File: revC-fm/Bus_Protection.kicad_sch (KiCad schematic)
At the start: 79 parts, among them Q24 MMDT2907AQ-7-F, Q25 MMDT5551-7-F, Q26 MMDT5551-7-F, Q27 MMDT5551-7-F, Q28 MMDT5551-7-F, Q29 MMDT2907AQ-7-F, Q30 BSS138DWQ-7, Q31 BSS138DWQ-7, Q32 BSS138DWQ-7, Q33 BSS138DWQ-7, Q34 MMDT3946, Q34 MMDT5551-7-F, Q35 MMDT5551-7-F, Q37 BSS138DWQ-7, Q38 BSS138DWQ-7

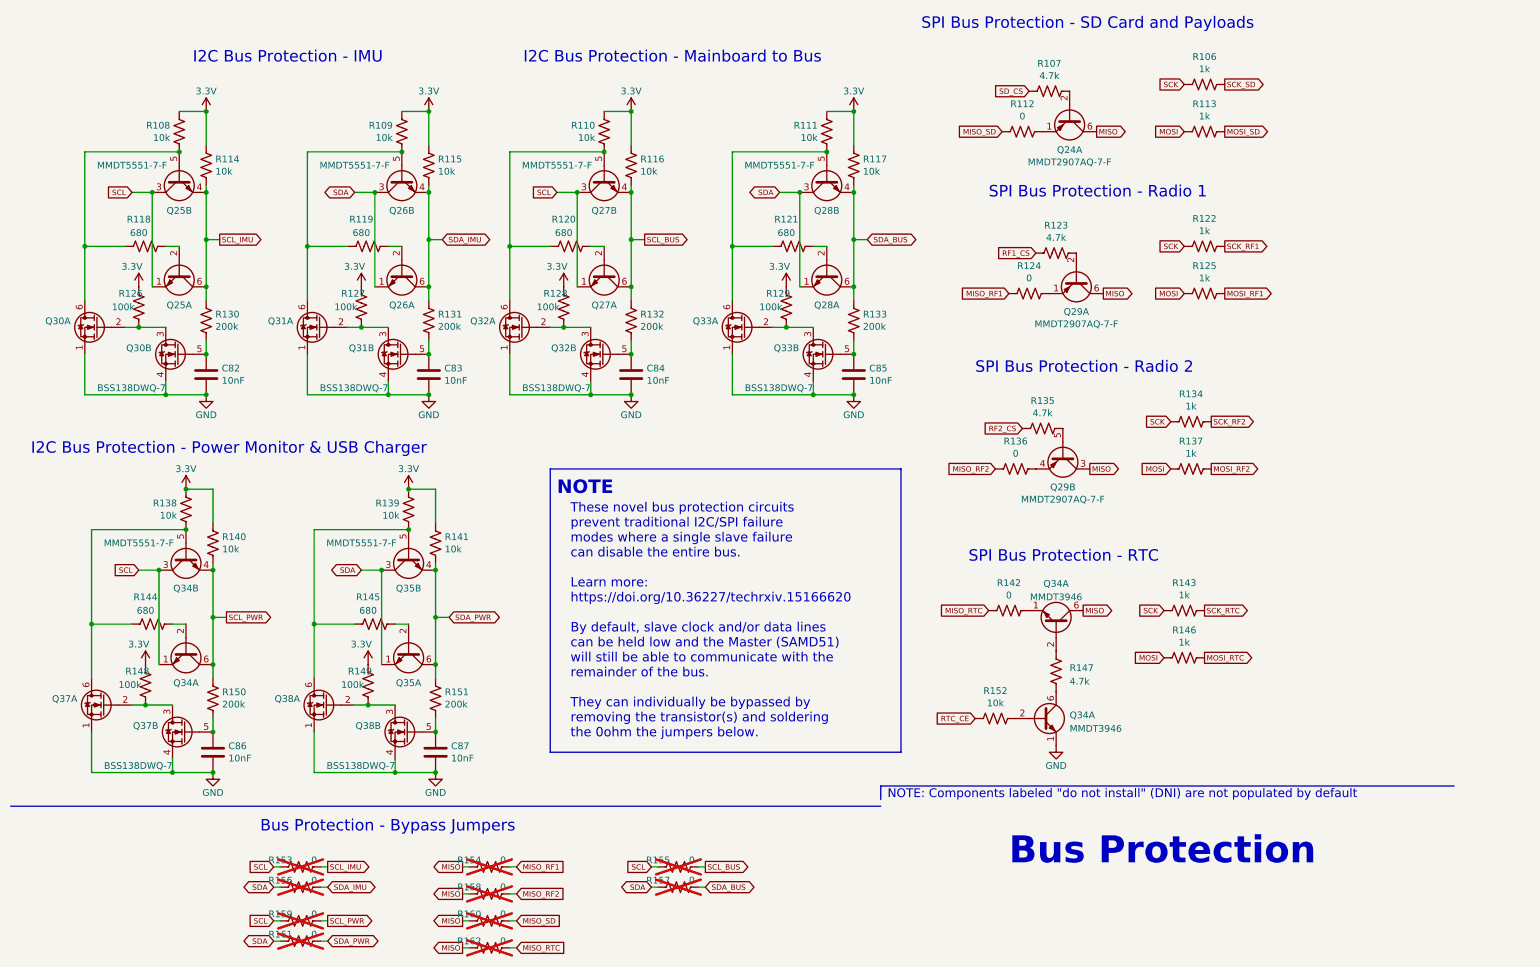
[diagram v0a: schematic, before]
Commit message: working revC
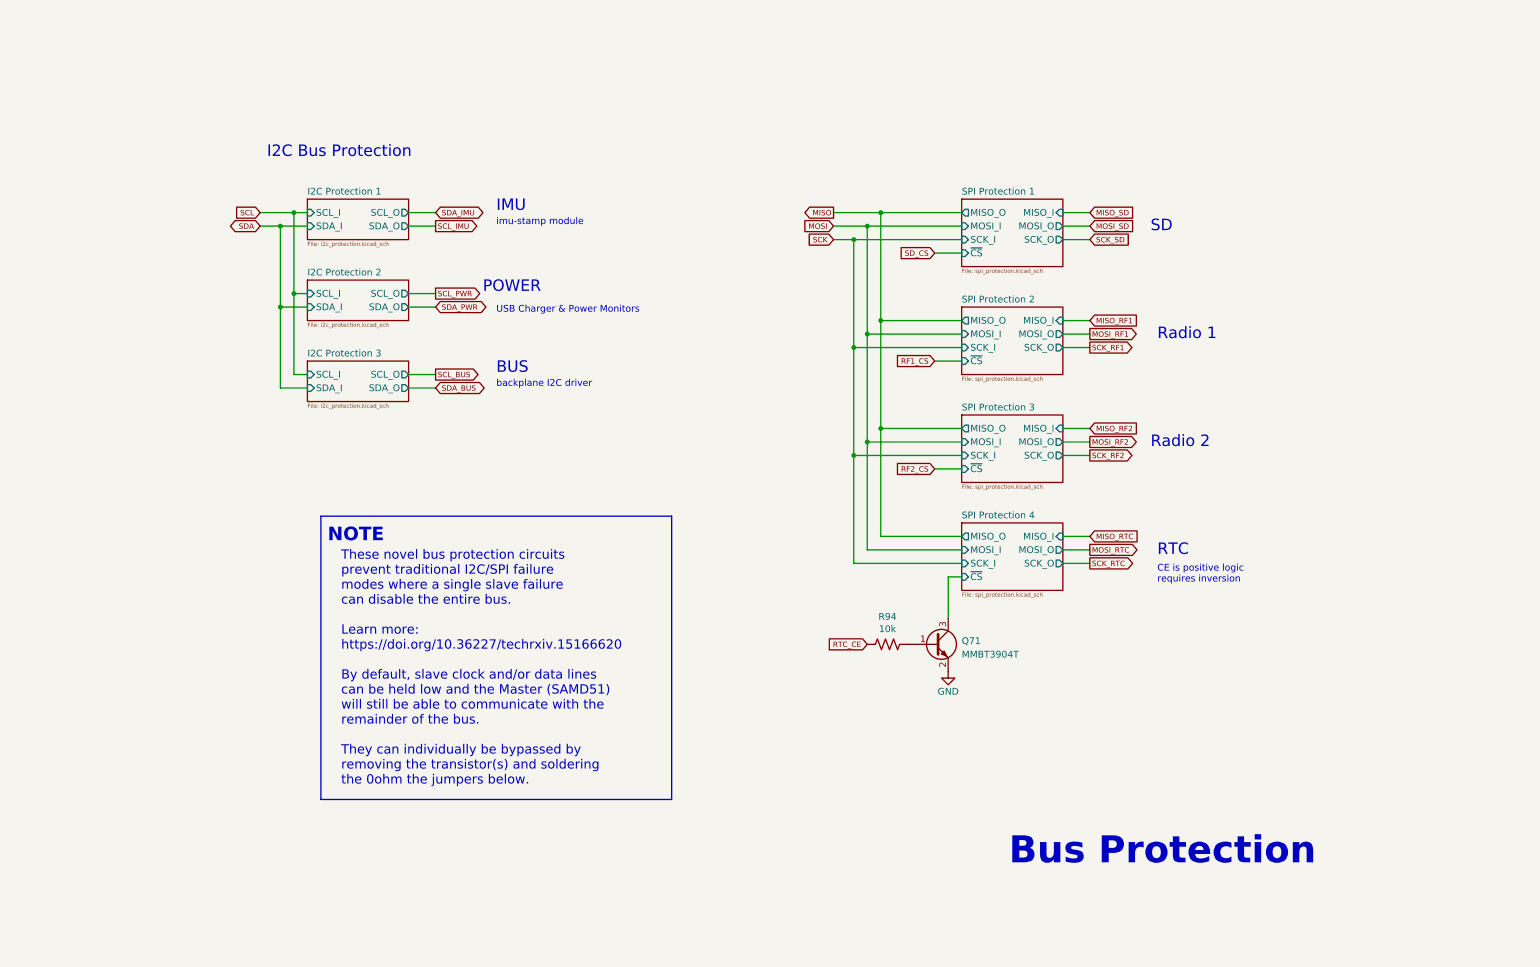
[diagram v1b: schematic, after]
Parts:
- removed C82, C83, C84, C85, C86, C87: 10nF, Capacitor_SMD:C_0603_1608Metric, symbol Device:C
- removed Q24, Q29: MMDT2907AQ-7-F, Package_TO_SOT_SMD:SOT-363_SC-70-6, symbol SierraLobo:MMDT2907
- removed Q25, Q26, Q27, Q28, Q34, Q35: MMDT5551-7-F, Package_TO_SOT_SMD:SOT-363_SC-70-6, symbol Transistor_BJT:MMDT5551
- removed Q30, Q31, Q32, Q33, Q37, Q38: BSS138DWQ-7, Package_TO_SOT_SMD:SOT-363_SC-70-6, symbol SierraLobo:BSS138DW
- removed R106, R113, R122, R125, R134, R137, R143, R146: 1k, Resistor_SMD:R_0603_1608Metric, symbol Device:R_US
- removed R107, R123, R135, R147: 4.7k, Resistor_SMD:R_0603_1608Metric, symbol Device:R_US
- removed R108, R109, R110, R111, R114, R115, R116, R117, R138, R139, R140, R141, R152: 10k, Resistor_SMD:R_0603_1608Metric, symbol Device:R_US
- removed R112, R124, R136, R142, R153, R154, R155, R156, R157, R158, R159, R160, R161, R162: 0, Resistor_SMD:R_0603_1608Metric, symbol Device:R_US
- removed R118, R119, R120, R121, R144, R145: 680, Resistor_SMD:R_0603_1608Metric, symbol Device:R_US
- removed R126, R127, R128, R129, R148, R149: 100k, Resistor_SMD:R_0603_1608Metric, symbol Device:R_US
- removed R130, R131, R132, R133, R150, R151: 200k, Resistor_SMD:R_0603_1608Metric, symbol Device:R_US
- added Q71: MMBT3904T, Package_TO_SOT_SMD:SOT-523, symbol Device:Q_NPN_BEC
- added R94: 10k, Resistor_SMD:R_0402_1005Metric, symbol Device:R_US
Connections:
- net GND: now also Q71.2 (E)
- net RTC_CE: now also R94.2
- new net: Q71.1 (B), R94.1
- new net SPI Protection 4/~{CS}: Q71.3 (C)
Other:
- added sheet I2C Protection 1 (i2c_protection.kicad_sch)
- added sheet I2C Protection 2 (i2c_protection.kicad_sch)
- added sheet I2C Protection 3 (i2c_protection.kicad_sch)
- added sheet SPI Protection 1 (spi_protection.kicad_sch)
- added sheet SPI Protection 2 (spi_protection.kicad_sch)
- added sheet SPI Protection 3 (spi_protection.kicad_sch)
- added sheet SPI Protection 4 (spi_protection.kicad_sch)
- note added: "BUS"
- note added: "CE is positive logic requires inversion"
- note added: "I2C Bus Protection"
- note added: "IMU"
- note added: "POWER"
- note added: "RTC"
- note added: "Radio 1"
- note added: "Radio 2"
- note added: "SD"
- note added: "USB Charger & Power Monitors"
- note added: "backplane I2C driver"
- note added: "imu-stamp module"
- note removed: "Bus Protection - Bypass Jumpers"
- note removed: "I2C Bus Protection - IMU"
- note removed: "I2C Bus Protection - Mainboard to Bus"
- note removed: "I2C Bus Protection - Power Monitor & USB Charger"
- note removed: "NOTE: Components labeled "do not install" (DNI) are not populated by default"
- note removed: "SPI Bus Protection - RTC"
- note removed: "SPI Bus Protection - Radio 1"
- note removed: "SPI Bus Protection - Radio 2"
- note removed: "SPI Bus Protection - SD Card and Payloads"
